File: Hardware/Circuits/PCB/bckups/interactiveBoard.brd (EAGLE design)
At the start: 72 x 150.1 mm, 65 parts, among them SW1 219-10, SW2 B3F-1000, SW3 B3F-1000, SW4 B3F-1000, SW5 B3F-1000, SW6 B3F-1000, SW7 B3F-1000, SW8 B3F-1000, SW9 B3F-1000

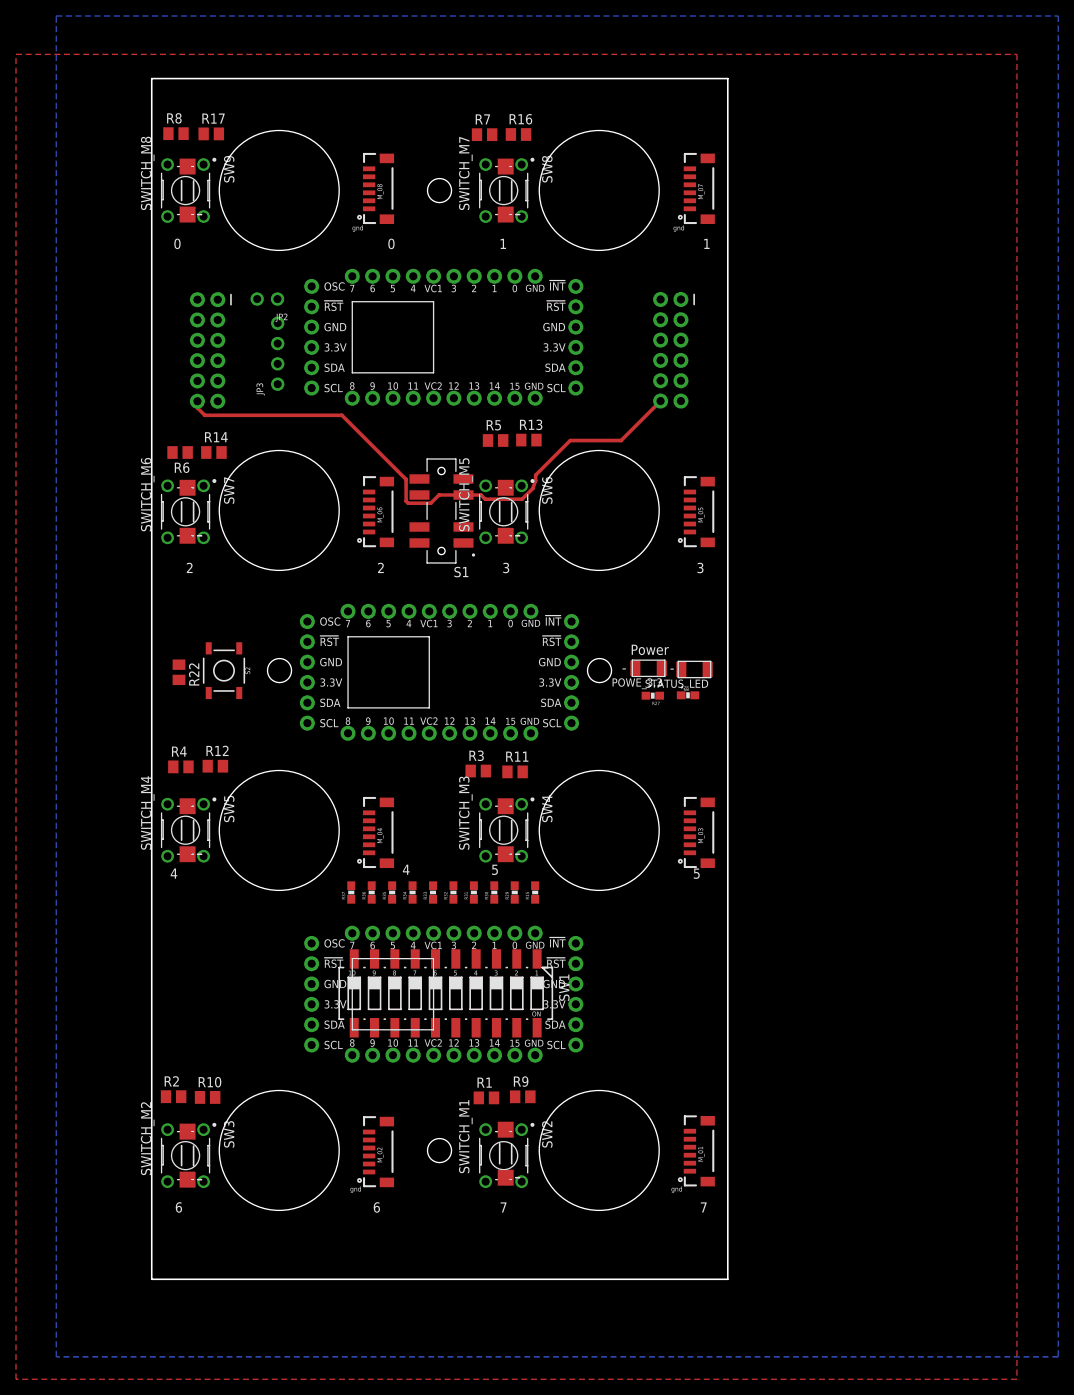
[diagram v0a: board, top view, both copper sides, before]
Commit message: clean circuit
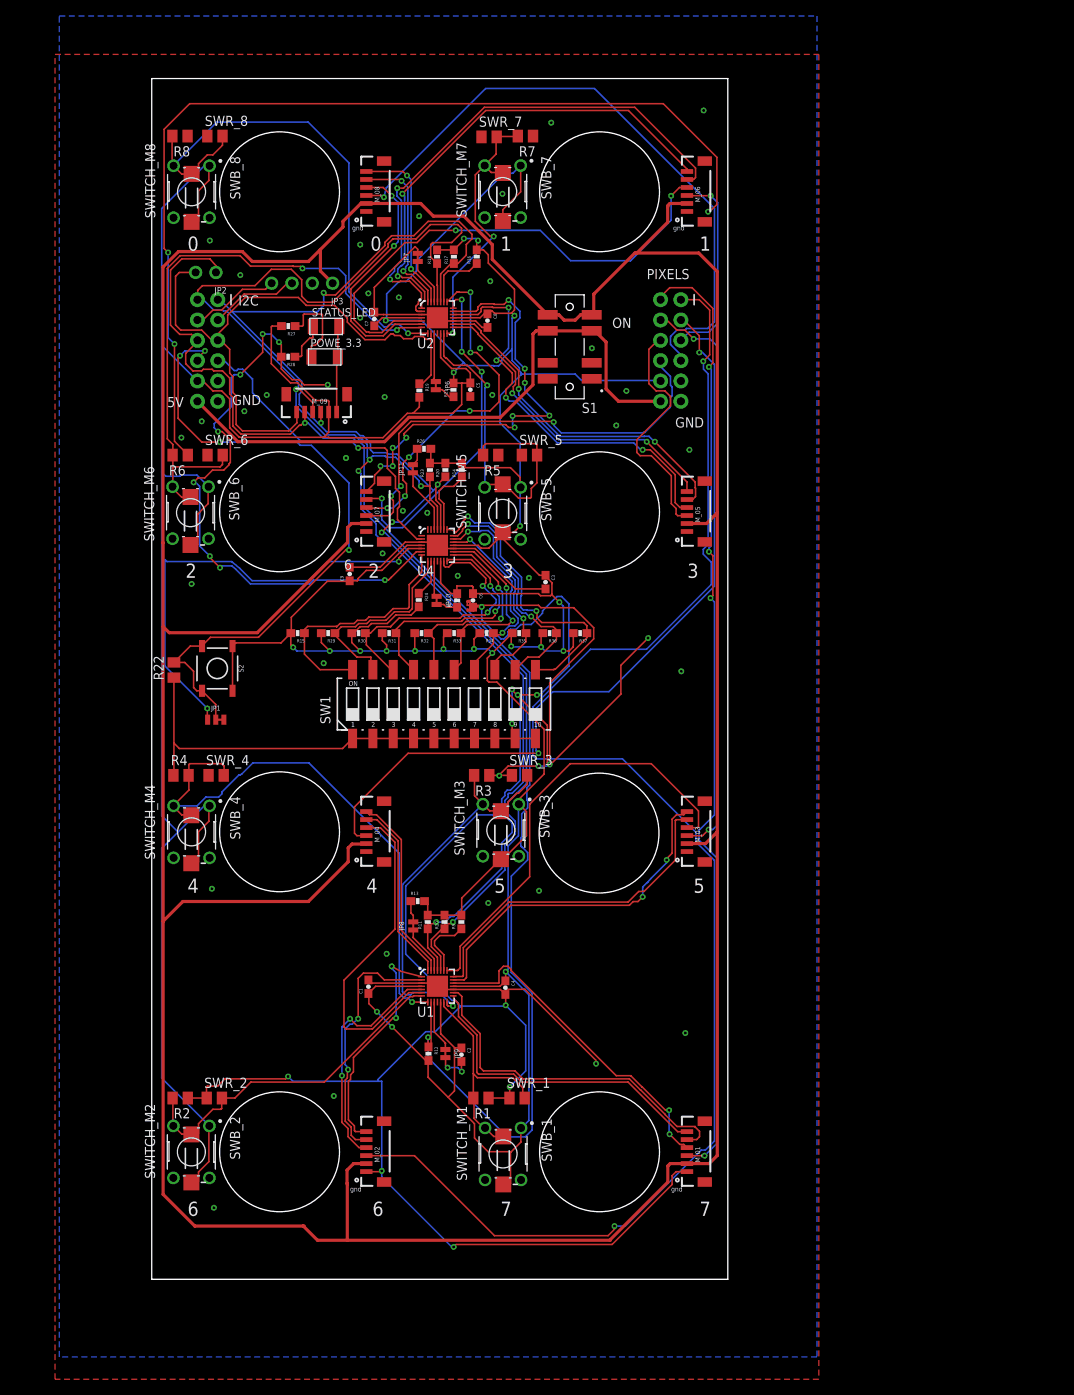
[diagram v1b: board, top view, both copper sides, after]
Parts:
- removed CONN01, CONN02: 2X6 FEMALE, SparkFun-Connectors:2X6
- removed SW2, SW3, SW4, SW5, SW6, SW7, SW8, SW9: B3F-1000, Switch:B3F-1000
- removed U$1, U$2, U$3: SX1509HOLE, SX1509_s:SX1509_HOLE
- added C1, C2, C3, C4, C5, C6, C7, C8, C9: 0.1uF, SparkFun-Capacitors:0603-CAP
- added J1, J2: 2X6 FEMALE, SparkFun-Connectors:2X6
- added JP1: JUMPER-SMT_3_1-NC_TRACE_NO-SILK, SparkFun-Jumpers:SMT-JUMPER_3_1-NC_TRACE_NO-SILK
- added JP10, JP11, JP6, JP7, JP8, JP9: JUMPER-SMT_2_NC_TRACE_NO-SILK, SparkFun-Jumpers:SMT-JUMPER_2_NC_TRACE_NO-SILK
- added M_09: (no value), SparkFun-Connectors:1X06-1MM
- added R18, R19, R20, R21, R23, R24, R25, R26: 10K, SparkFun-Resistors:0603-RES
- added SWB_1, SWB_2, SWB_3, SWB_4, SWB_5, SWB_6, SWB_7, SWB_8: B3F-1000, Switch:B3F-1000
- added SWR_1, SWR_2, SWR_3, SWR_4, SWR_5, SWR_6, SWR_7, SWR_8: 10K, resistor:M0805
- added U1, U2, U4: SX1509, SparkFun-DigitalIC:QFN-28
- R10, R11, R12, R13, R14, R16, R17, R9: device resistor:M0805 -> SparkFun-Resistors:0603-RES
- moved R28 65.5 mm to (17.4, 115.3), turned to 180 degrees
- moved R27 64.9 mm to (17.4, 119.1)
- moved STATUS_LED 62.9 mm to (22.1, 119.0), turned to 0 degrees
- moved R13 59.3 mm to (33.6, 47.2)
- moved M_07 57.1 mm to (28.4, 96.0)
- moved M_06 56.4 mm to (68.5, 136.0)
- moved POWE_3.3 56.2 mm to (22.0, 115.2), turned to 0 degrees
- moved R12 44.7 mm to (34.9, 28.1), turned to 270 degrees
- moved R15 44.0 mm to (18.6, 80.7), turned to 180 degrees
- moved R37 43.2 mm to (53.9, 80.7), turned to 180 degrees
- moved R29 39.9 mm to (22.4, 80.7), turned to 180 degrees
- moved R36 39.3 mm to (50.1, 80.7), turned to 180 degrees
- moved R10 36.9 mm to (37.0, 44.6), turned to 90 degrees
- moved R30 36.6 mm to (26.2, 80.7), turned to 180 degrees
- moved SW1 36.2 mm to (36.9, 71.9), turned to 0 degrees
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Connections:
- removed net N$1: S1.7
- removed net N$25: U$3.INT
- new net !INT_SX3: R24.1, U4.9
- new net !RESET_SX1: R9.1, U1.23
- new net !RESET_SX2: R16.1, U2.23
- new net !RESET_SX3: R14.1, U4.23
- new net ADDR0_SX1: JP8.1, U1.26
- new net ADDR0_SX2: JP7.1, U2.26
- new net ADDR0_SX3: JP11.1, U4.26
- new net ADDR1_SX1: JP9.1, U1.10
- new net ADDR1_SX2: JP6.1, U2.10
- new net ADDR1_SX3: JP10.1, U4.10
- new net N$14: JP10.2, R25.1
- new net N$15: JP11.2, R26.1
- new net N$5: JP6.2, R21.1
- new net N$8: JP8.2, R13.1
- new net OSCIO_SX1: U1.11
- new net OSCIO_SX2: U2.11
- new net OSCIO_SX3: U4.11
- new net RESET: J1.8, JP1.2, JP1.3, R22.2, S2.3, S2.4
- net 0_SX1: now also U1.27; no longer U$1.0
- net 0_SX2: now also U2.27; no longer U$2.0
- net 0_SX3: now also U4.27; no longer U$3.0
- net 10_SX1: now also U1.15; no longer U$1.10
- net 10_SX2: now also U2.15; no longer U$2.10
- net 10_SX3: now also R32.1, SW1.16, U4.15; no longer R33.1, SW1.15, U$3.10
- net 11_SX1: now also U1.16; no longer U$1.11
- net 11_SX2: now also U2.16; no longer U$2.11
- net 11_SX3: now also R33.1, SW1.15, U4.16; no longer R34.1, SW1.14, U$3.11
- net 12_SX1: now also U1.19; no longer U$1.12
- net 12_SX2: now also U2.19; no longer U$2.12
- net 12_SX3: now also R34.1, SW1.14, U4.19; no longer R35.1, SW1.13, U$3.12
- net 13_SX1: now also U1.20; no longer U$1.13
- net 13_SX2: now also U2.20; no longer U$2.13
- net 13_SX3: now also R35.1, SW1.13, U4.20; no longer R36.1, SW1.12, U$3.13
- net 14_SX1: now also U1.21; no longer U$1.14
- net 14_SX2: now also U2.21; no longer U$2.14
- net 14_SX3: now also R36.1, SW1.12, U4.21; no longer R37.1, SW1.11, U$3.14
- net 15_SX1: now also U1.22; no longer U$1.15
- net 15_SX2: now also U2.22; no longer U$2.15
- net 15_SX3: now also R37.1, SW1.11, U4.22; no longer R28.2, U$3.15
- net 1_SX1: now also U1.28; no longer U$1.1
- net 1_SX2: now also U2.28; no longer U$2.1
- net 1_SX3: now also U4.28; no longer U$3.1
- net 2_SX1: now also U1.1; no longer U$1.2
- net 2_SX2: now also U2.1; no longer U$2.2
- net 2_SX3: now also U4.1; no longer CONN01.8, U$3.2
- net 3.3V: now also C1.1, C2.1, C3.1, C4.1, C5.1, C6.1, C7.1, C8.1, C9.1, J1.10, J2.10, M_09.2, R10.2, R11.2, R12.2, R13.2, R14.2, R16.2, R17.2, R18.2, R19.2, R20.2, R21.2, R23.2, R24.2, R25.2, R26.2, R9.2, SWB_1.1, SWB_2.1, SWB_3.1, SWB_4.1, SWB_5.1, SWB_6.1, SWB_7.1, SWB_8.1, U1.12, U1.18, U1.4, U2.12, U2.18, U2.4, U4.12, U4.18, U4.4; no longer CONN01.10, CONN02.10, JP3.1, SW2.1, SW3.1, SW4.1, SW5.1, SW6.1, SW7.1, SW8.1, SW9.1, U$1.3.3V, U$1.3.3V_2, U$2.3.3V, U$2.3.3V_2, U$3.3.3V, U$3.3.3V_2
- net 3_SX1: now also U1.2; no longer U$1.3
- net 3_SX2: now also U2.2; no longer U$2.3
- net 3_SX3: now also J1.7, U4.2; no longer CONN01.7, U$3.3
- net 4_SX1: now also U1.5; no longer U$1.4
- net 4_SX2: now also U2.5; no longer U$2.4
- net 4_SX3: now also JP1.1, U4.5; no longer R22.2, S2.3, S2.4, U$3.4
- net 5_SX1: now also U1.6; no longer U$1.5
- net 5_SX2: now also U2.6; no longer U$2.5
- net 5_SX3: now also R28.2, U4.6; no longer R15.1, SW1.20, U$3.5
- net 6_SX1: now also SWB_2.3, SWR_2.2, U1.7; no longer R10.2, SW3.3, U$1.6
- net 6_SX2: now also SWB_6.3, SWR_6.2, U2.7; no longer R14.2, SW7.3, U$2.6
- net 6_SX3: now also R15.1, SW1.20, U4.7; no longer R29.1, SW1.19, U$3.6
- net 7_SX1: now also SWB_4.3, SWR_4.2, U1.8; no longer R12.2, SW5.3, U$1.7
- net 7_SX2: now also SWB_8.3, SWR_8.2, U2.8; no longer R17.2, SW9.3, U$2.7
- net 7_SX3: now also R29.1, SW1.19, U4.8; no longer R30.1, SW1.18, U$3.7
- net 8_SX1: now also SWB_1.3, SWR_1.2, U1.13; no longer R9.2, SW2.3, U$1.8
- net 8_SX2: now also SWB_5.3, SWR_5.2, U2.13; no longer R13.2, SW6.3, U$2.8
- net 8_SX3: now also R30.1, SW1.18, U4.13; no longer R31.1, SW1.17, U$3.8
- net 9_SX1: now also SWB_3.3, SWR_3.2, U1.14; no longer R11.2, SW4.3, U$1.9
- net 9_SX2: now also SWB_7.3, SWR_7.2, U2.14; no longer R16.2, SW8.3, U$2.9
- net 9_SX3: now also R31.1, SW1.17, U4.14; no longer R32.1, SW1.16, U$3.9
- net CAN_RX2: now also J1.4; no longer CONN01.4, JP2.2
- net CAN_TX2: now also J1.3; no longer CONN01.3, JP2.1
- net GND_MCU: now also C1.2, C2.2, C3.2, C4.2, C5.2, C6.2, C7.2, C8.2, C9.2, J1.11, J1.9, J2.11, J2.9, JP7.2, JP9.2, M_09.1, SWR_1.1, SWR_2.1, SWR_3.1, SWR_4.1, SWR_5.1, SWR_6.1, SWR_7.1, SWR_8.1, U1.17, U1.29, U1.3, U2.17, U2.29, U2.3, U4.17, U4.29, U4.3; no longer CONN01.11, CONN01.9, CONN02.11, CONN02.9, R10.1, R11.1, R12.1, R13.1, R14.1, R16.1, R17.1, R9.1, U$1.GND, U$1.GND_1, U$1.GND_2, U$1.GND_3, U$2.GND, U$2.GND_1, U$2.GND_2, U$2.GND_3, U$3.GND, U$3.GND_1, U$3.GND_2, U$3.GND_3
- net INT_01: now also J1.6, JP2.1, M_09.5, R12.1, U1.9; no longer CONN01.6, U$1.INT
- net INT_02: now also J1.5, JP2.2, M_09.6, R19.1, U2.9; no longer CONN01.5, U$2.INT
- net NEOPIXEL_01: now also J2.2; no longer CONN02.2
- net NEOPIXEL_02: now also J2.1; no longer CONN02.1
- net NEOPIXEL_03: now also J2.4; no longer CONN02.4
- net NEOPIXEL_04: now also J2.3; no longer CONN02.3
- net NEOPIXEL_05: now also J2.6; no longer CONN02.6
- net NEOPIXEL_06: now also J2.5; no longer CONN02.5
- net NEOPIXEL_07: now also J2.8; no longer CONN02.8
- net NEOPIXEL_08: now also J2.7; no longer CONN02.7
- net SCL_00: now also J1.2, M_09.4, R11.1, R18.1, R23.1, U1.25, U2.25, U4.25; no longer CONN01.2, U$1.SCL, U$1.SCL_2, U$2.SCL, U$2.SCL_2, U$3.SCL, U$3.SCL_2
- net SDA_00: now also J1.1, M_09.3, R10.1, R17.1, R20.1, U1.24, U2.24, U4.24; no longer CONN01.1, U$1.SDA, U$1.SDA_2, U$2.SDA, U$2.SDA_2, U$3.SDA, U$3.SDA_2
- net VCC_5V: now also JP3.1, S1.4
- net VCC_5V_IN: now also J1.12, J2.12, S1.7; no longer CONN01.12, CONN02.12
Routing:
- net 3.3V: track 0.00 -> 718.7 mm, vias 0 -> 21
- net GND_MCU: track 0.00 -> 581.9 mm, vias 0 -> 58
- net VCC_5V: track 0.00 -> 488.7 mm
- net NEOPIXEL_02: track 0.00 -> 191.1 mm, vias 0 -> 2
- net SCL_00: track 0.00 -> 190.0 mm, vias 0 -> 5
- net INT_01: track 0.00 -> 178.6 mm, vias 0 -> 2
- net SDA_00: track 0.00 -> 174.8 mm, vias 0 -> 6
- net NEOPIXEL_01: track 0.00 -> 120.0 mm, vias 0 -> 4
- net NEOPIXEL_04: track 0.00 -> 100.5 mm, vias 0 -> 2
- net RESET: track 0.00 -> 85.3 mm, vias 0 -> 4
- net NEOPIXEL_08: track 0.00 -> 80.0 mm, vias 0 -> 1
- net 5_SX3: track 0.00 -> 78.5 mm, vias 0 -> 9
- net INT_02: track 0.00 -> 77.3 mm
- net 6_SX2: track 0.00 -> 75.8 mm, vias 0 -> 2
- net NEOPIXEL_03: track 0.00 -> 72.7 mm, vias 0 -> 2
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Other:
- outline, holes or cut-outs redrawn
- board text added: "ON"
- board text added: "PIXELS"
- board text removed: "-"
- board text removed: "3.3V"
- board text removed: "NEO"
- board text removed: "Power"
- board text removed: "SX_01"
- board text removed: "SX_02"
- board text removed: "SX_03"
